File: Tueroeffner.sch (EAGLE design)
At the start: 34 parts, among them IC1 NCP1117ST33T3G, IC3 M25PE20, K2 EC2-12TNU, Q1 2N7002CK, Q2 2N7002CK

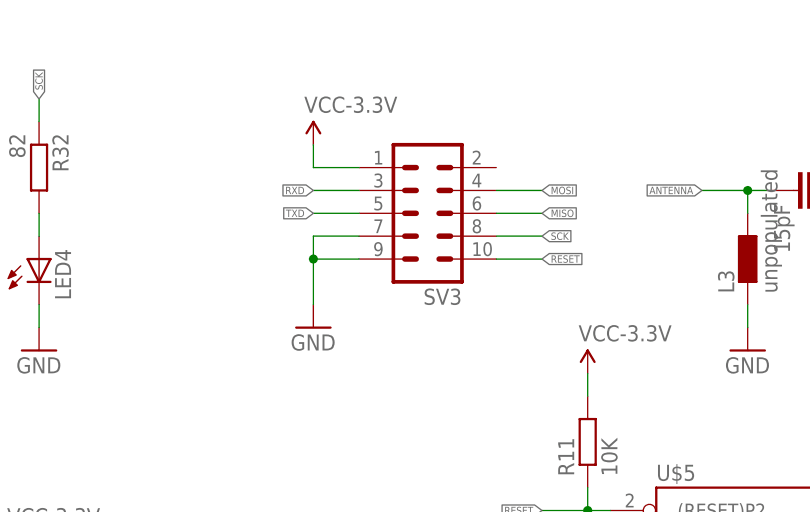
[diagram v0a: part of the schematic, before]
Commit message: RC candidate
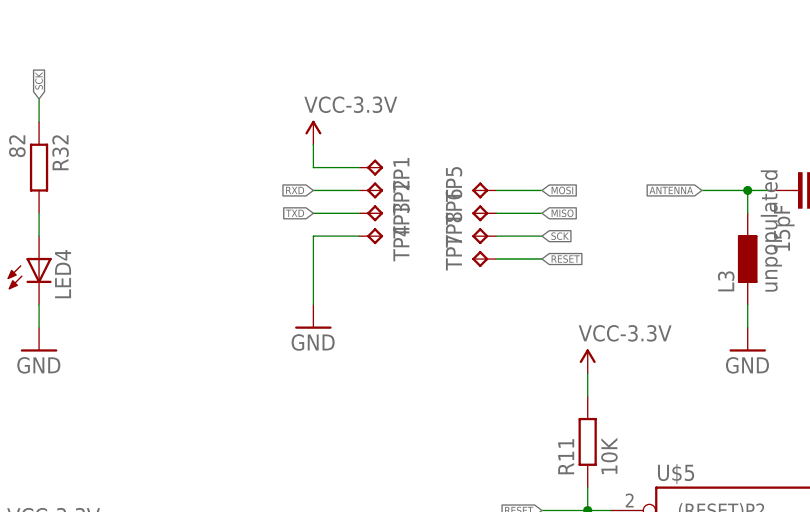
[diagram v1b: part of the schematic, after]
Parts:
- removed SV3: (no value), con-lstb:MA05-2
- added TP1, TP2, TP3, TP4, TP5, TP6, TP7, TP8: TPB1,27, testpad:TPB1,27
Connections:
- net GND: now also TP4.TP; no longer SV3.7, SV3.9
- net MISO: now also TP6.TP; no longer SV3.6
- net MOSI: now also TP5.TP; no longer SV3.4
- net RESET: now also TP7.TP; no longer SV3.10
- net RXD: now also TP2.TP; no longer SV3.3
- net SCK: now also TP8.TP; no longer SV3.8
- net TXD: now also TP3.TP; no longer SV3.5
- net VCC-3.3V: now also TP1.TP; no longer SV3.1
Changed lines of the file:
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@@
 <part name="GND1" library="SparkFun-Aesthetics" deviceset="GND" device=""/>
 <part name="3.3V2" library="SparkFun-Aesthetics" deviceset="VCC" device="" value="VCC-3.3V"/>
-<part name="SV3" library="con-lstb" deviceset="MA05-2" device=""/>
 <part name="R11" library="resistor" deviceset="R-EU_" device="M2012" value="10K"/>
 <part name="3.3V8" library="SparkFun-Aesthetics" deviceset="VCC" device="" value="VCC-3.3V"/>
@@
 <part name="GND5" library="supply1" deviceset="GND" device=""/>
 <part name="5-12V2" library="SparkFun-Aesthetics" deviceset="VCC" device="" value="VCC-5-12V"/>
+<part name="TP1" library="testpad" deviceset="TP" device="B1,27"/>
+<part name="TP2" library="testpad" deviceset="TP" device="B1,27"/>
+<part name="TP3" library="testpad" deviceset="TP" device="B1,27"/>
+<part name="TP4" library="testpad" deviceset="TP" device="B1,27"/>
+<part name="TP5" library="testpad" deviceset="TP" device="B1,27"/>
+<part name="TP6" library="testpad" deviceset="TP" device="B1,27"/>
+<part name="TP7" library="testpad" deviceset="TP" device="B1,27"/>
+<part name="TP8" library="testpad" deviceset="TP" device="B1,27"/>
 </parts>
 <sheets>
@@
 <instance part="GND1" gate="1" x="177.8" y="15.24"/>
 <instance part="3.3V2" gate="G$1" x="177.8" y="35.56"/>
-<instance part="SV3" gate="G$1" x="162.56" y="76.2" rot="R180"/>
 <instance part="R11" gate="G$1" x="180.34" y="50.8" rot="R90"/>
 <instance part="3.3V8" gate="G$1" x="180.34" y="58.42"/>
@@
 <instance part="GND5" gate="1" x="320.04" y="17.78"/>
 <instance part="5-12V2" gate="G$1" x="304.8" y="45.72"/>
+<instance part="TP1" gate="G$1" x="157.48" y="81.28" rot="R270"/>
+<instance part="TP2" gate="G$1" x="157.48" y="78.74" rot="R270"/>
+<instance part="TP3" gate="G$1" x="157.48" y="76.2" rot="R270"/>
+<instance part="TP4" gate="G$1" x="157.48" y="73.66" rot="R270"/>
+<instance part="TP5" gate="G$1" x="167.64" y="78.74" rot="R90"/>
+<instance part="TP6" gate="G$1" x="167.64" y="76.2" rot="R90"/>
+<instance part="TP7" gate="G$1" x="167.64" y="71.12" rot="R90"/>
+<instance part="TP8" gate="G$1" x="167.64" y="73.66" rot="R90"/>
 </instances>
 <busses>
@@
 </segment>
 <segment>
-<pinref part="SV3" gate="G$1" pin="7"/>
+<pinref part="GND6" gate="1" pin="GND"/>
 <wire x1="154.94" y1="73.66" x2="149.86" y2="73.66" width="0.1524" layer="91"/>
-<pinref part="GND6" gate="1" pin="GND"/>
-<wire x1="149.86" y1="66.04" x2="149.86" y2="71.12" width="0.1524" layer="91"/>
-<pinref part="SV3" gate="G$1" pin="9"/>
-<wire x1="149.86" y1="71.12" x2="149.86" y2="73.66" width="0.1524" layer="91"/>
-<wire x1="154.94" y1="71.12" x2="149.86" y2="71.12" width="0.1524" layer="91"/>
-<junction x="149.86" y="71.12"/>
+<wire x1="149.86" y1="66.04" x2="149.86" y2="73.66" width="0.1524" layer="91"/>
+<pinref part="TP4" gate="G$1" pin="TP"/>
 </segment>
 <segment>
@@
 </segment>
 <segment>
-<pinref part="SV3" gate="G$1" pin="1"/>
+<pinref part="3.3V9" gate="G$1" pin="VCC"/>
 <wire x1="154.94" y1="81.28" x2="149.86" y2="81.28" width="0.1524" layer="91"/>
-<pinref part="3.3V9" gate="G$1" pin="VCC"/>
 <wire x1="149.86" y1="81.28" x2="149.86" y2="83.82" width="0.1524" layer="91"/>
+<pinref part="TP1" gate="G$1" pin="TP"/>
 </segment>
 <segment>
@@
 </segment>
 <segment>
-<pinref part="SV3" gate="G$1" pin="5"/>
+<label x="149.86" y="76.2" size="0.8128" layer="95" rot="R180" xref="yes"/>
+<pinref part="TP3" gate="G$1" pin="TP"/>
 <wire x1="154.94" y1="76.2" x2="149.86" y2="76.2" width="0.1524" layer="91"/>
-<label x="149.86" y="76.2" size="0.8128" layer="95" rot="R180" xref="yes"/>
 </segment>
 </net>
@@
 </segment>
 <segment>
-<pinref part="SV3" gate="G$1" pin="3"/>
+<label x="149.86" y="78.74" size="0.8128" layer="95" rot="R180" xref="yes"/>
+<pinref part="TP2" gate="G$1" pin="TP"/>
 <wire x1="154.94" y1="78.74" x2="149.86" y2="78.74" width="0.1524" layer="91"/>
-<label x="149.86" y="78.74" size="0.8128" layer="95" rot="R180" xref="yes"/>
 </segment>
 </net>
@@
 </segment>
 <segment>
-<pinref part="SV3" gate="G$1" pin="10"/>
+<label x="175.26" y="71.12" size="0.8128" layer="95" ratio="7" xref="yes"/>
+<pinref part="TP7" gate="G$1" pin="TP"/>
 <wire x1="170.18" y1="71.12" x2="175.26" y2="71.12" width="0.1524" layer="91"/>
-<label x="175.26" y="71.12" size="0.8128" layer="95" ratio="7" xref="yes"/>
 </segment>
 </net>
@@
 </segment>
 <segment>
-<pinref part="SV3" gate="G$1" pin="4"/>
+<label x="175.26" y="78.74" size="0.8128" layer="95" ratio="7" xref="yes"/>
+<pinref part="TP5" gate="G$1" pin="TP"/>
 <wire x1="170.18" y1="78.74" x2="175.26" y2="78.74" width="0.1524" layer="91"/>
-<label x="175.26" y="78.74" size="0.8128" layer="95" ratio="7" xref="yes"/>
 </segment>
 <segment>
@@
 </segment>
 <segment>
-<pinref part="SV3" gate="G$1" pin="8"/>
+<label x="175.26" y="73.66" size="0.8128" layer="95" ratio="7" xref="yes"/>
+<pinref part="TP8" gate="G$1" pin="TP"/>
 <wire x1="170.18" y1="73.66" x2="175.26" y2="73.66" width="0.1524" layer="91"/>
-<label x="175.26" y="73.66" size="0.8128" layer="95" ratio="7" xref="yes"/>
 </segment>
 <segment>
@@
 </segment>
 <segment>
-<pinref part="SV3" gate="G$1" pin="6"/>
+<label x="175.26" y="76.2" size="0.8128" layer="95" ratio="7" xref="yes"/>
+<pinref part="TP6" gate="G$1" pin="TP"/>
 <wire x1="170.18" y1="76.2" x2="175.26" y2="76.2" width="0.1524" layer="91"/>
-<label x="175.26" y="76.2" size="0.8128" layer="95" ratio="7" xref="yes"/>
-</segment>
-<segment>
+</segment>
+<segment>

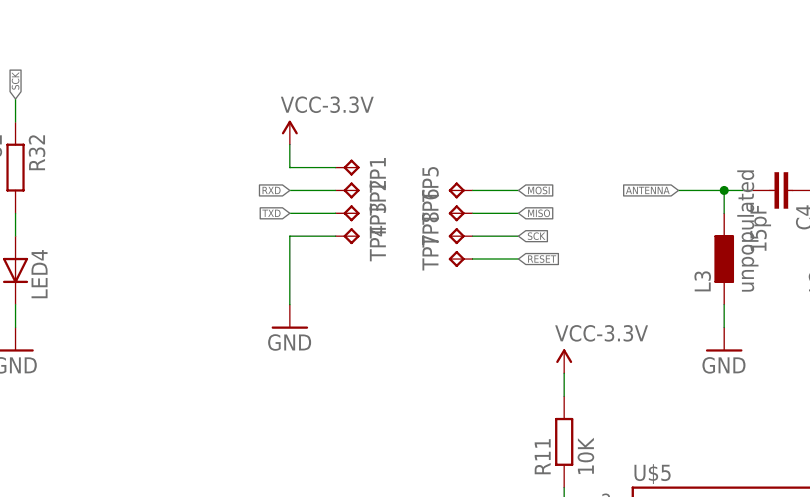
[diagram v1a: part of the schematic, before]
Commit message: Clean Up
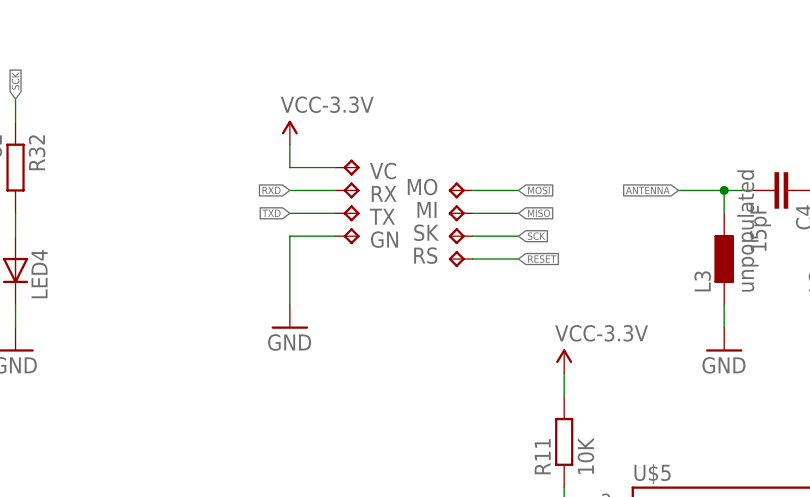
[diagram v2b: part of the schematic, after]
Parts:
- renumbered TP1 to VC, TP2 to RX, TP3 to TX, TP4 to GN, TP5 to MO, TP6 to MI, TP7 to RS, TP8 to SK
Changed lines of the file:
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@@
 <part name="GND5" library="supply1" deviceset="GND" device=""/>
 <part name="5-12V2" library="SparkFun-Aesthetics" deviceset="VCC" device="" value="VCC-5-12V"/>
-<part name="TP1" library="testpad" deviceset="TP" device="B1,27"/>
-<part name="TP2" library="testpad" deviceset="TP" device="B1,27"/>
-<part name="TP3" library="testpad" deviceset="TP" device="B1,27"/>
-<part name="TP4" library="testpad" deviceset="TP" device="B1,27"/>
-<part name="TP5" library="testpad" deviceset="TP" device="B1,27"/>
-<part name="TP6" library="testpad" deviceset="TP" device="B1,27"/>
-<part name="TP7" library="testpad" deviceset="TP" device="B1,27"/>
-<part name="TP8" library="testpad" deviceset="TP" device="B1,27"/>
+<part name="VC" library="testpad" deviceset="TP" device="B1,27"/>
+<part name="RX" library="testpad" deviceset="TP" device="B1,27"/>
+<part name="TX" library="testpad" deviceset="TP" device="B1,27"/>
+<part name="GN" library="testpad" deviceset="TP" device="B1,27"/>
+<part name="MO" library="testpad" deviceset="TP" device="B1,27"/>
+<part name="MI" library="testpad" deviceset="TP" device="B1,27"/>
+<part name="RS" library="testpad" deviceset="TP" device="B1,27"/>
+<part name="SK" library="testpad" deviceset="TP" device="B1,27"/>
 </parts>
 <sheets>
@@
 <instance part="GND5" gate="1" x="320.04" y="17.78"/>
 <instance part="5-12V2" gate="G$1" x="304.8" y="45.72"/>
-<instance part="TP1" gate="G$1" x="157.48" y="81.28" rot="R270"/>
-<instance part="TP2" gate="G$1" x="157.48" y="78.74" rot="R270"/>
-<instance part="TP3" gate="G$1" x="157.48" y="76.2" rot="R270"/>
-<instance part="TP4" gate="G$1" x="157.48" y="73.66" rot="R270"/>
-<instance part="TP5" gate="G$1" x="167.64" y="78.74" rot="R90"/>
-<instance part="TP6" gate="G$1" x="167.64" y="76.2" rot="R90"/>
-<instance part="TP7" gate="G$1" x="167.64" y="71.12" rot="R90"/>
-<instance part="TP8" gate="G$1" x="167.64" y="73.66" rot="R90"/>
+<instance part="VC" gate="G$1" x="157.48" y="81.28" smashed="yes" rot="R270">
+<attribute name="NAME" x="158.75" y="80.01" size="1.778" layer="95"/>
+<attribute name="TP_SIGNAL_NAME" x="156.21" y="80.01" size="1.778" layer="97" rot="R270"/>
+</instance>
+<instance part="RX" gate="G$1" x="157.48" y="78.74" smashed="yes" rot="R270">
+<attribute name="NAME" x="158.75" y="77.47" size="1.778" layer="95"/>
+<attribute name="TP_SIGNAL_NAME" x="156.21" y="77.47" size="1.778" layer="97" rot="R270"/>
+</instance>
+<instance part="TX" gate="G$1" x="157.48" y="76.2" smashed="yes" rot="R270">
+<attribute name="NAME" x="158.75" y="74.93" size="1.778" layer="95"/>
+<attribute name="TP_SIGNAL_NAME" x="156.21" y="74.93" size="1.778" layer="97" rot="R270"/>
+</instance>
+<instance part="GN" gate="G$1" x="157.48" y="73.66" smashed="yes" rot="R270">
+<attribute name="NAME" x="158.75" y="72.39" size="1.778" layer="95"/>
+<attribute name="TP_SIGNAL_NAME" x="156.21" y="72.39" size="1.778" layer="97" rot="R270"/>
+</instance>
+<instance part="MO" gate="G$1" x="167.64" y="78.74" smashed="yes" rot="R90">
+<attribute name="NAME" x="166.37" y="80.01" size="1.778" layer="95" rot="R180"/>
+<attribute name="TP_SIGNAL_NAME" x="168.91" y="80.01" size="1.778" layer="97" rot="R90"/>
+</instance>
+<instance part="MI" gate="G$1" x="167.64" y="76.2" smashed="yes" rot="R90">
+<attribute name="NAME" x="166.37" y="77.47" size="1.778" layer="95" rot="R180"/>
+<attribute name="TP_SIGNAL_NAME" x="168.91" y="77.47" size="1.778" layer="97" rot="R90"/>
+</instance>
+<instance part="RS" gate="G$1" x="167.64" y="71.12" smashed="yes" rot="R90">
+<attribute name="NAME" x="166.37" y="72.39" size="1.778" layer="95" rot="R180"/>
+<attribute name="TP_SIGNAL_NAME" x="168.91" y="72.39" size="1.778" layer="97" rot="R90"/>
+</instance>
+<instance part="SK" gate="G$1" x="167.64" y="73.66" smashed="yes" rot="R90">
+<attribute name="NAME" x="166.37" y="74.93" size="1.778" layer="95" rot="R180"/>
+<attribute name="TP_SIGNAL_NAME" x="168.91" y="74.93" size="1.778" layer="97" rot="R90"/>
+</instance>
 </instances>
 <busses>
@@
 <wire x1="154.94" y1="73.66" x2="149.86" y2="73.66" width="0.1524" layer="91"/>
 <wire x1="149.86" y1="66.04" x2="149.86" y2="73.66" width="0.1524" layer="91"/>
-<pinref part="TP4" gate="G$1" pin="TP"/>
+<pinref part="GN" gate="G$1" pin="TP"/>
 </segment>
 <segment>
@@
 <wire x1="154.94" y1="81.28" x2="149.86" y2="81.28" width="0.1524" layer="91"/>
 <wire x1="149.86" y1="81.28" x2="149.86" y2="83.82" width="0.1524" layer="91"/>
-<pinref part="TP1" gate="G$1" pin="TP"/>
+<pinref part="VC" gate="G$1" pin="TP"/>
 </segment>
 <segment>
@@
 <segment>
 <label x="149.86" y="76.2" size="0.8128" layer="95" rot="R180" xref="yes"/>
-<pinref part="TP3" gate="G$1" pin="TP"/>
+<pinref part="TX" gate="G$1" pin="TP"/>
 <wire x1="154.94" y1="76.2" x2="149.86" y2="76.2" width="0.1524" layer="91"/>
 </segment>
@@
 <segment>
 <label x="149.86" y="78.74" size="0.8128" layer="95" rot="R180" xref="yes"/>
-<pinref part="TP2" gate="G$1" pin="TP"/>
+<pinref part="RX" gate="G$1" pin="TP"/>
 <wire x1="154.94" y1="78.74" x2="149.86" y2="78.74" width="0.1524" layer="91"/>
 </segment>
@@
 <segment>
 <label x="175.26" y="71.12" size="0.8128" layer="95" ratio="7" xref="yes"/>
-<pinref part="TP7" gate="G$1" pin="TP"/>
+<pinref part="RS" gate="G$1" pin="TP"/>
 <wire x1="170.18" y1="71.12" x2="175.26" y2="71.12" width="0.1524" layer="91"/>
 </segment>
@@
 <segment>
 <label x="175.26" y="78.74" size="0.8128" layer="95" ratio="7" xref="yes"/>
-<pinref part="TP5" gate="G$1" pin="TP"/>
+<pinref part="MO" gate="G$1" pin="TP"/>
 <wire x1="170.18" y1="78.74" x2="175.26" y2="78.74" width="0.1524" layer="91"/>
 </segment>
@@
 <segment>
 <label x="175.26" y="73.66" size="0.8128" layer="95" ratio="7" xref="yes"/>
-<pinref part="TP8" gate="G$1" pin="TP"/>
+<pinref part="SK" gate="G$1" pin="TP"/>
 <wire x1="170.18" y1="73.66" x2="175.26" y2="73.66" width="0.1524" layer="91"/>
 </segment>
@@
 <segment>
 <label x="175.26" y="76.2" size="0.8128" layer="95" ratio="7" xref="yes"/>
-<pinref part="TP6" gate="G$1" pin="TP"/>
+<pinref part="MI" gate="G$1" pin="TP"/>
 <wire x1="170.18" y1="76.2" x2="175.26" y2="76.2" width="0.1524" layer="91"/>
 </segment>
